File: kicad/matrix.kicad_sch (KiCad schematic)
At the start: 108 parts, among them SW401 SW_Push_45deg, SW402 SW_Push_45deg, SW403 SW_Push_45deg, SW404 SW_Push_45deg, SW405 SW_Push_45deg, SW406 SW_Push_45deg, SW407 SW_Push_45deg, SW408 SW_Push_45deg, SW409 SW_Push_45deg, SW410 SW_Push_45deg, SW411 SW_Push_45deg, SW412 SW_Push_45deg, SW413 SW_Push_45deg, SW414 SW_Push_45deg, SW415 SW_Push_45deg, SW416 SW_Push_45deg, SW417 SW_Push_45deg, SW418 SW_Push_45deg, SW419 SW_Push_45deg, SW420 SW_Push_45deg, SW421 SW_Push_45deg, SW422 SW_Push_45deg, SW423 SW_Push_45deg, SW424 SW_Push_45deg, SW425 SW_Push_45deg, SW426 SW_Push_45deg, SW427 SW_Push_45deg, SW428 SW_Push_45deg, SW429 SW_Push_45deg, SW430 SW_Push_45deg, SW431 SW_Push_45deg, SW432 SW_Push_45deg, SW433 SW_Push_45deg, SW434 SW_Push_45deg, SW435 SW_Push_45deg, SW436 SW_Push_45deg, SW437 SW_Push_45deg, SW438 SW_Push_45deg, SW439 SW_Push_45deg, SW440 SW_Push_45deg, SW441 SW_Push_45deg, SW442 SW_Push_45deg, SW443 SW_Push_45deg, SW444 SW_Push_45deg, SW445 SW_Push_45deg, SW446 SW_Push_45deg, SW447 SW_Push_45deg, SW448 SW_Push_45deg, SW449 SW_Push_45deg, SW450 SW_Push_45deg, SW451 SW_Push_45deg, SW452 SW_Push_45deg, SW453 SW_Push_45deg, SW454 SW_Push_45deg

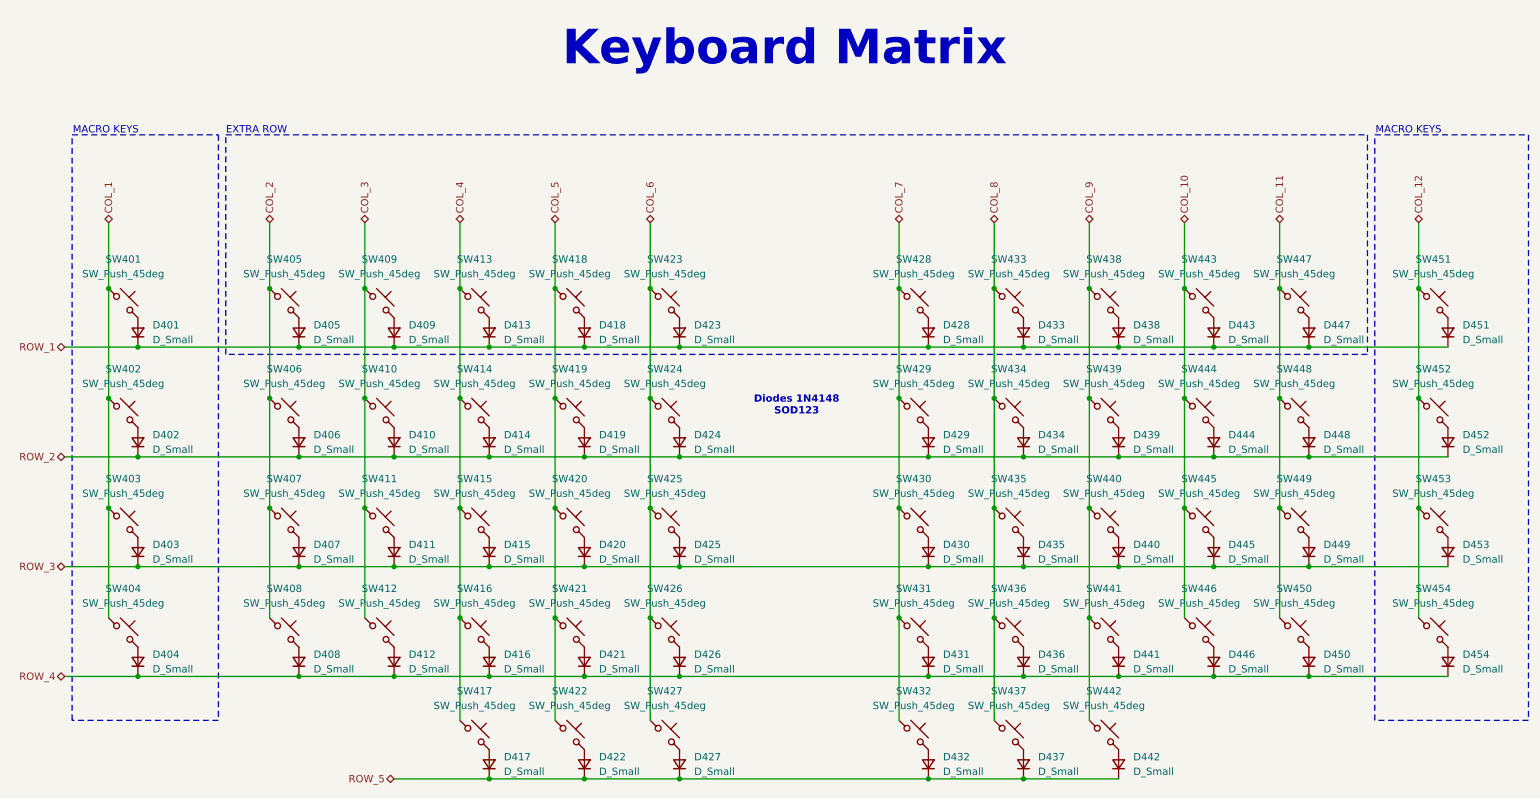
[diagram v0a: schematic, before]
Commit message: moved to revision b
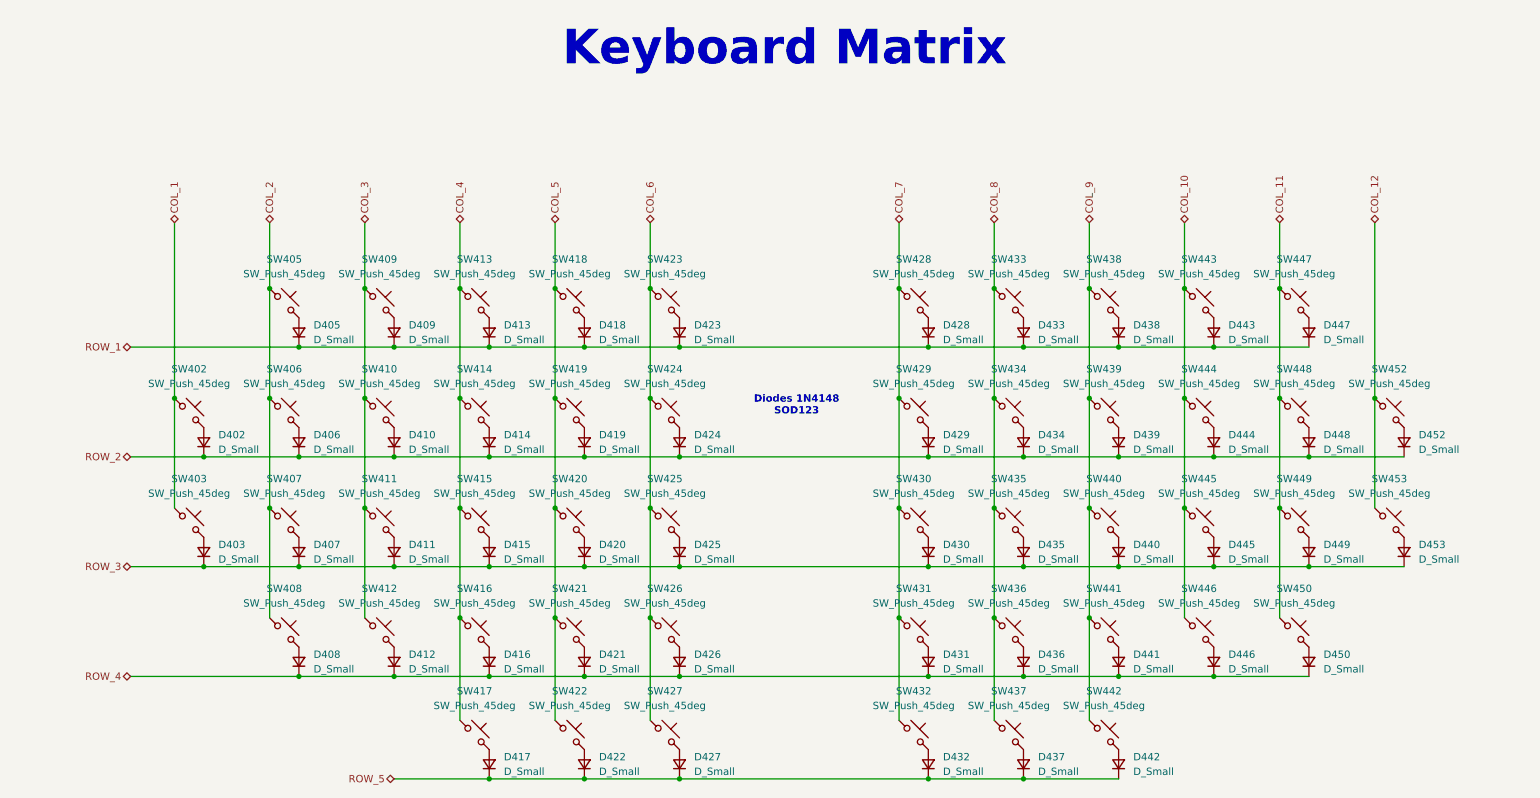
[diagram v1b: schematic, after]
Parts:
- removed D401, D404, D451, D454: D_Small, Diode_SMD:D_SOD-123, symbol Device:D_Small
- removed SW401, SW404, SW451, SW454: SW_Push_45deg, Button_Switch_Keyboard:SW_Cherry_MX_1.00u_PCB, symbol Switch:SW_Push_45deg
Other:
- note removed: "EXTRA ROW"
- note removed: "MACRO KEYS"
- moved on the sheet: D402, D403, D452, D453, SW402, SW403, SW452, SW453
